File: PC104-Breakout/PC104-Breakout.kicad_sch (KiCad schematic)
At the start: 21 parts, among them J1 Screw_Terminal_01x02, J2 Screw_Terminal_01x02, J3 Screw_Terminal_01x02, M1 MountingHole_Pad, M2 MountingHole_Pad, M3 MountingHole_Pad, M4 MountingHole_Pad, M5 MountingHole_Pad, M6 MountingHole_Pad, M7 MountingHole_Pad, M8 MountingHole_Pad

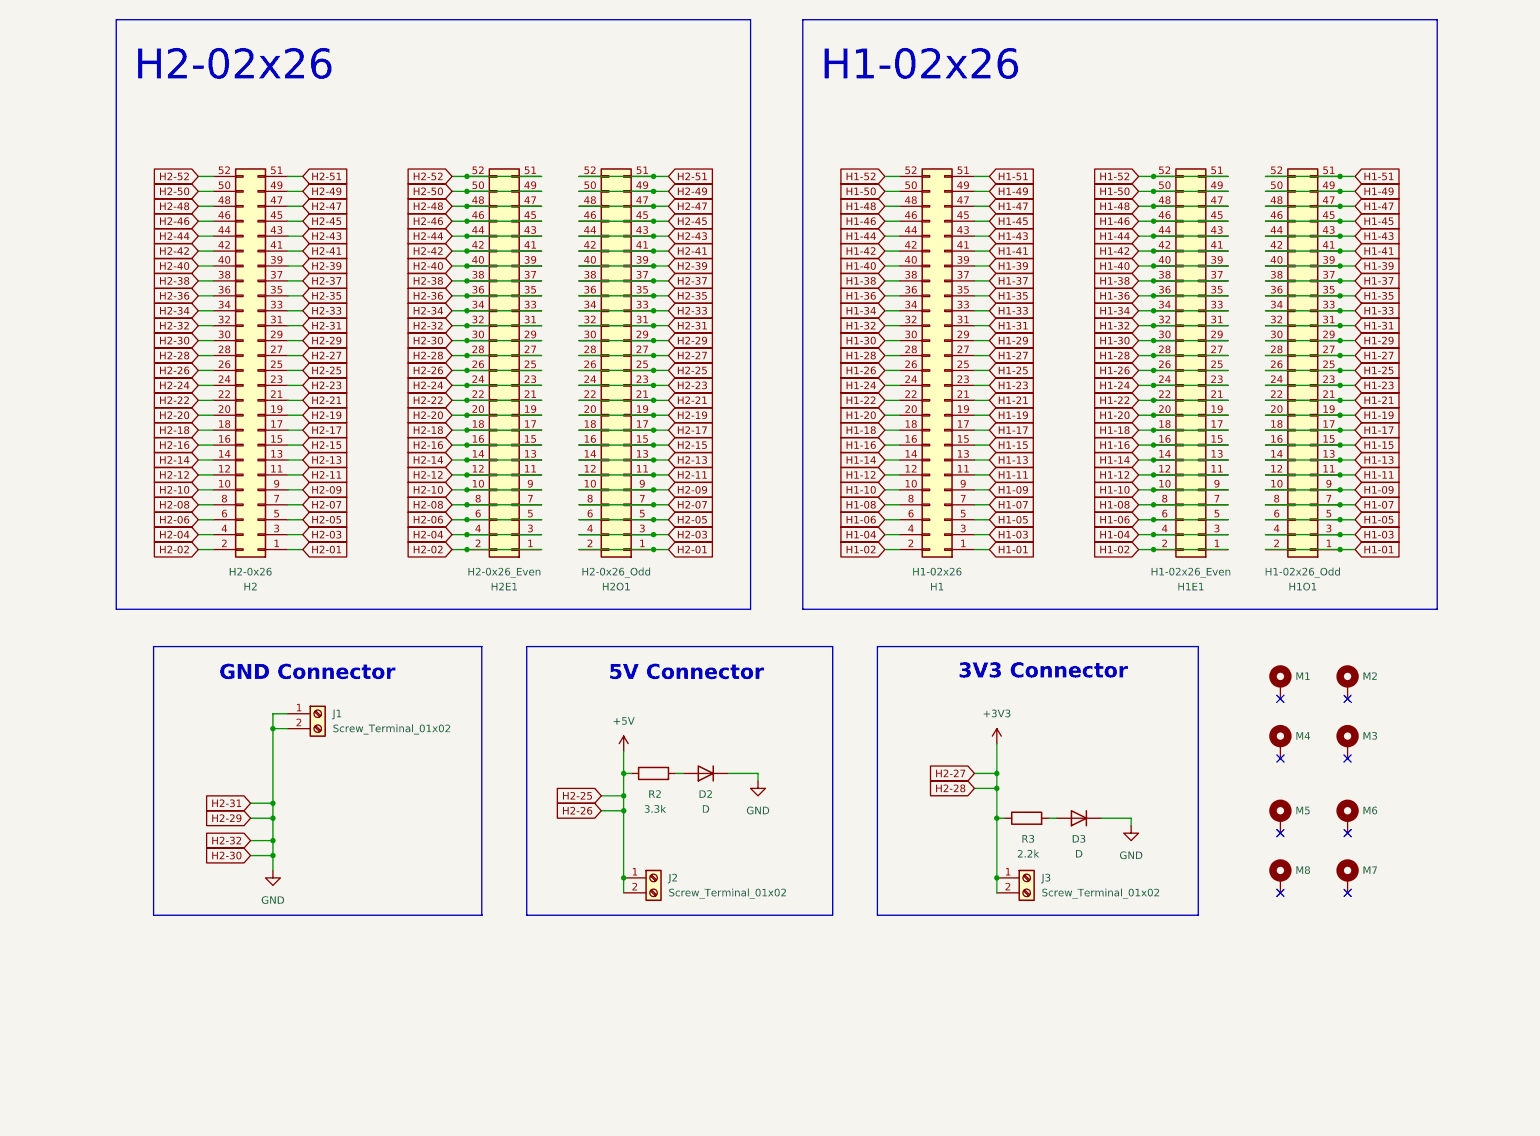
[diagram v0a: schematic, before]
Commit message: Update for Rev 3, do layout
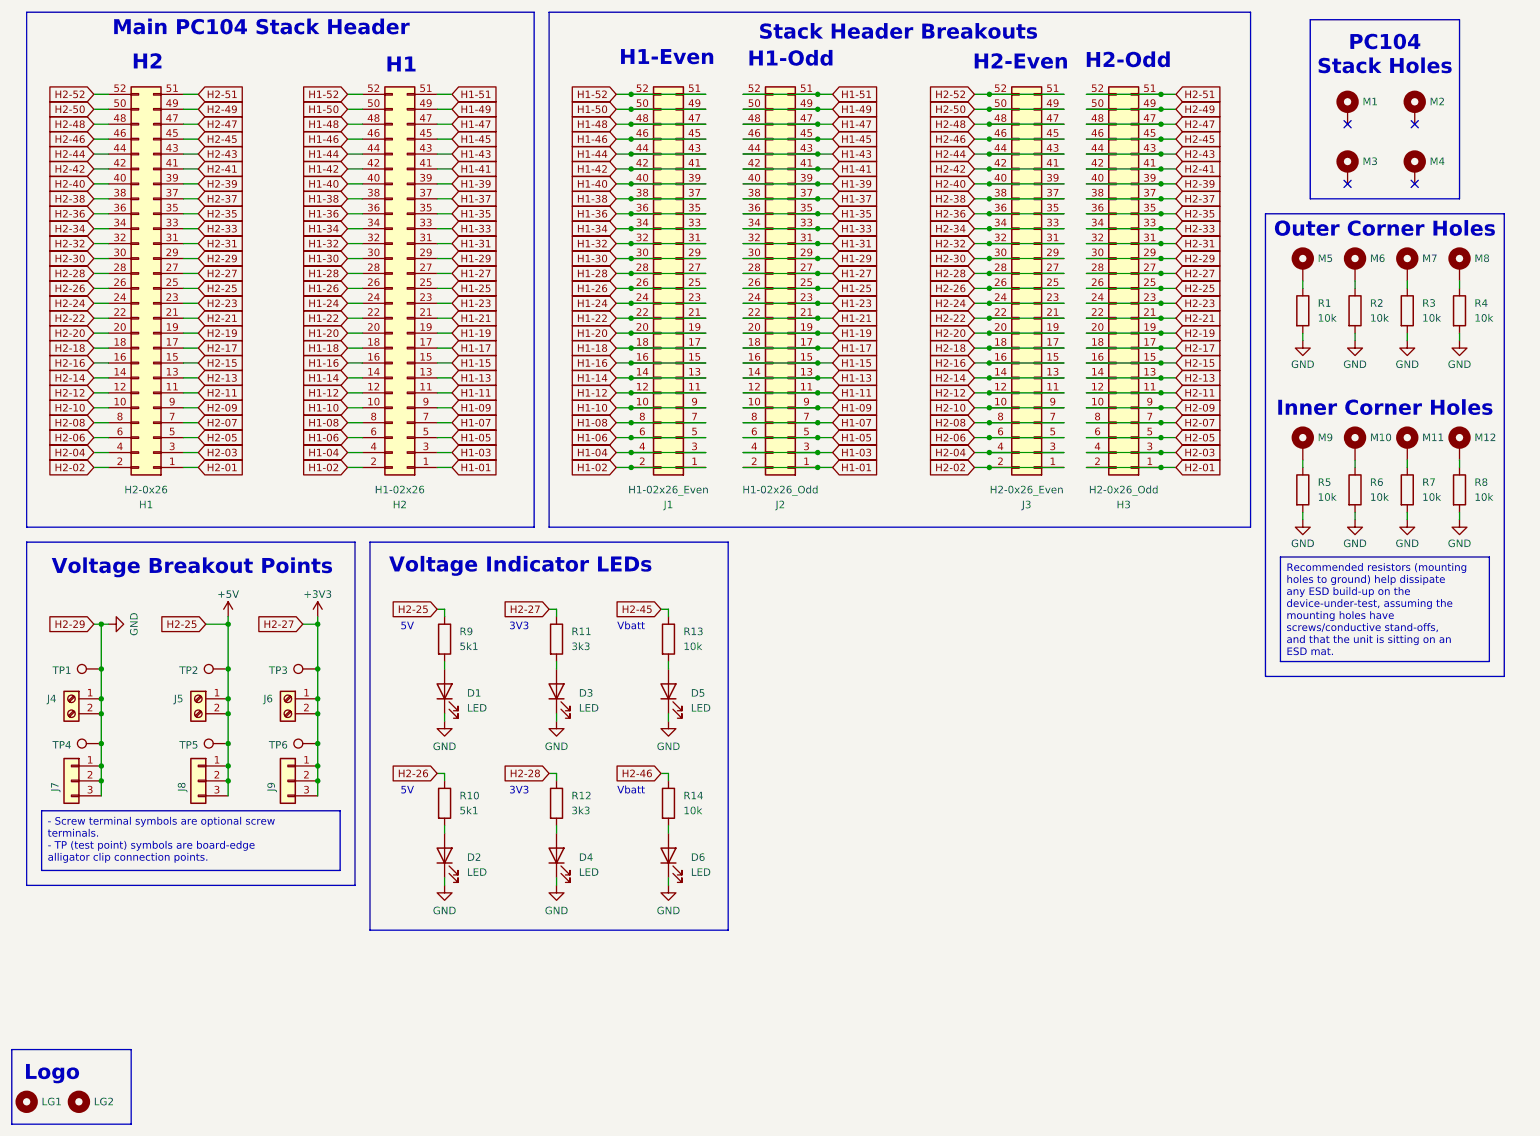
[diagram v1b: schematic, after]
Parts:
- removed D2, D3: D, Diode_SMD:D_1206_3216Metric_Pad1.42x1.75mm_HandSolder, symbol Device:D
- removed J1, J2, J3: Screw_Terminal_01x02, TerminalBlock:TerminalBlock_bornier-2_P5.08mm, symbol Connector:Screw_Terminal_01x02
- added D1, D2, D3, D4, D5, D6: LED, LED_SMD:LED_0603_1608Metric_Pad1.05x0.95mm_HandSolder, symbol Device:LED
- added J4, J5, J6: Screw_Terminal_01x02, TerminalBlock:TerminalBlock_bornier-2_P5.08mm, symbol Connector:Screw_Terminal_01x02
- added J7, J8, J9: Conn_01x02, Connector_PinHeader_2.54mm:PinHeader_1x03_P2.54mm_Vertical, symbol Connector_Generic:Conn_01x03
- added LG1, LG2: MountingHole, PC104-Breakout-Lib:CTS-Logo-50x25, symbol Mechanical:MountingHole
- added M10, M11, M12, M9: MountingHole_Pad, MountingHole:MountingHole_3.2mm_M3_Pad, symbol Mechanical:MountingHole_Pad
- added R1, R13, R14, R4, R5, R6, R7, R8: 10k, Resistor_SMD:R_0603_1608Metric_Pad0.98x0.95mm_HandSolder, symbol Device:R
- added R10, R9: 5k1, Resistor_SMD:R_0603_1608Metric_Pad0.98x0.95mm_HandSolder, symbol Device:R
- added R11, R12: 3k3, Resistor_SMD:R_0603_1608Metric_Pad0.98x0.95mm_HandSolder, symbol Device:R
- added TP1, TP2, TP3, TP4, TP5, TP6: TestPoint, PC104-Breakout-Lib:EdgeAlligatorConnector, symbol Connector:TestPoint
- R2: value 3.3k -> 10k; footprint Resistor_SMD:R_1206_3216Metric_Pad1.30x1.75mm_HandSolder -> Resistor_SMD:R_0603_1608Metric_Pad0.98x0.95mm_HandSolder
- R3: value 2.2k -> 10k; footprint Resistor_SMD:R_1206_3216Metric_Pad1.30x1.75mm_HandSolder -> Resistor_SMD:R_0603_1608Metric_Pad0.98x0.95mm_HandSolder
- renumbered H2 to H1, H1 to H2, H2O1 to H3, H1E1 to J1, H1O1 to J2, H2E1 to J3, M4 to M3, M3 to M4
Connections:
- net +3V3: now also J6.1 (Pin_1), J6.2 (Pin_2), J9.1 (Pin_1), J9.2 (Pin_2), J9.3 (Pin_3), R11.1, TP3.1, TP6.1; no longer H1.28 (Pin_28), J3.27 (Pin_27), J3.28 (Pin_28), R3.1
- net +5V: now also J5.1 (Pin_1), J5.2 (Pin_2), J8.1 (Pin_1), J8.2 (Pin_2), J8.3 (Pin_3), R9.1, TP2.1, TP5.1; no longer H1.26 (Pin_26), J3.25 (Pin_25), J3.26 (Pin_26), R2.1
- net GND: now also R2.2, R3.2, D1.1 (K), D2.1 (K), D3.1 (K), D4.1 (K), D5.1 (K), D6.1 (K), J4.1 (Pin_1), J4.2 (Pin_2), J7.1 (Pin_1), J7.2 (Pin_2), J7.3 (Pin_3), R1.2, R4.2, R5.2, R6.2, R7.2, R8.2, TP1.1, TP4.1; no longer H1.30 (Pin_30), H1.31 (Pin_31), H1.32 (Pin_32), H3.31 (Pin_31), H3.32 (Pin_32), J3.29 (Pin_29), J3.30 (Pin_30), J3.31 (Pin_31), J3.32 (Pin_32)
- net H2-45: now also R13.1
- net H2-46: now also R14.1
- net at M8.1: now also R4.1
- net at M5.1: now also R1.1
- net at M7.1: now also R3.1
- net at M6.1: now also R2.1
- new net: D1.2 (A), R9.2
- new net: M12.1, R8.1
- new net: D3.2 (A), R11.2
- new net: D4.2 (A), R12.2
- new net: M9.1, R5.1
- new net: D2.2 (A), R10.2
- new net: M11.1, R7.1
- new net: M10.1, R6.1
- new net: D5.2 (A), R13.2
- new net: D6.2 (A), R14.2
- new net H2-26: H1.26 (Pin_26), J3.25 (Pin_25), J3.26 (Pin_26), R10.1
- new net H2-28: H1.28 (Pin_28), J3.27 (Pin_27), J3.28 (Pin_28), R12.1
- new net H2-30: H1.30 (Pin_30), J3.29 (Pin_29), J3.30 (Pin_30)
- new net H2-31: H1.31 (Pin_31), H3.31 (Pin_31), H3.32 (Pin_32)
- new net H2-32: H1.32 (Pin_32), J3.31 (Pin_31), J3.32 (Pin_32)
- no-connect marks 8 -> 4
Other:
- note added: "3V3"
- note added: "5V"
- note added: "H1"
- note added: "H1-Even"
- note added: "H1-Odd"
- note added: "H2"
- note added: "H2-Even"
- note added: "H2-Odd"
- note added: "Inner Corner Holes"
- note added: "Logo"
- note added: "Main PC104 Stack Header"
- note added: "Outer Corner Holes"
- note added: "PC104 Stack Holes"
- note added: "Stack Header Breakouts"
- note added: "Vbatt"
- note added: "Voltage Breakout Points"
- note added: "Voltage Indicator LEDs"
- note removed: "3V3 Connector"
- note removed: "5V Connector"
- note removed: "GND Connector"
- note removed: "H1-02x26"
- note removed: "H2-02x26"
- moved on the sheet: H1, H2, H3, J1, J2, J3, M1, M2, M3, M4, M5, M6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
